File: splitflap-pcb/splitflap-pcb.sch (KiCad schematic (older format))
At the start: 21 parts, among them J1 INPUT CONN, J2 HALL 1, J3 HALL 2, J4 STEPPER 1, J5 STEPPER 2, J6 OUTPUT CONN, J7 AVR-ISP-6, U1 REGULATOR, U2 ATtiny88-AU, U3 TPIC6595

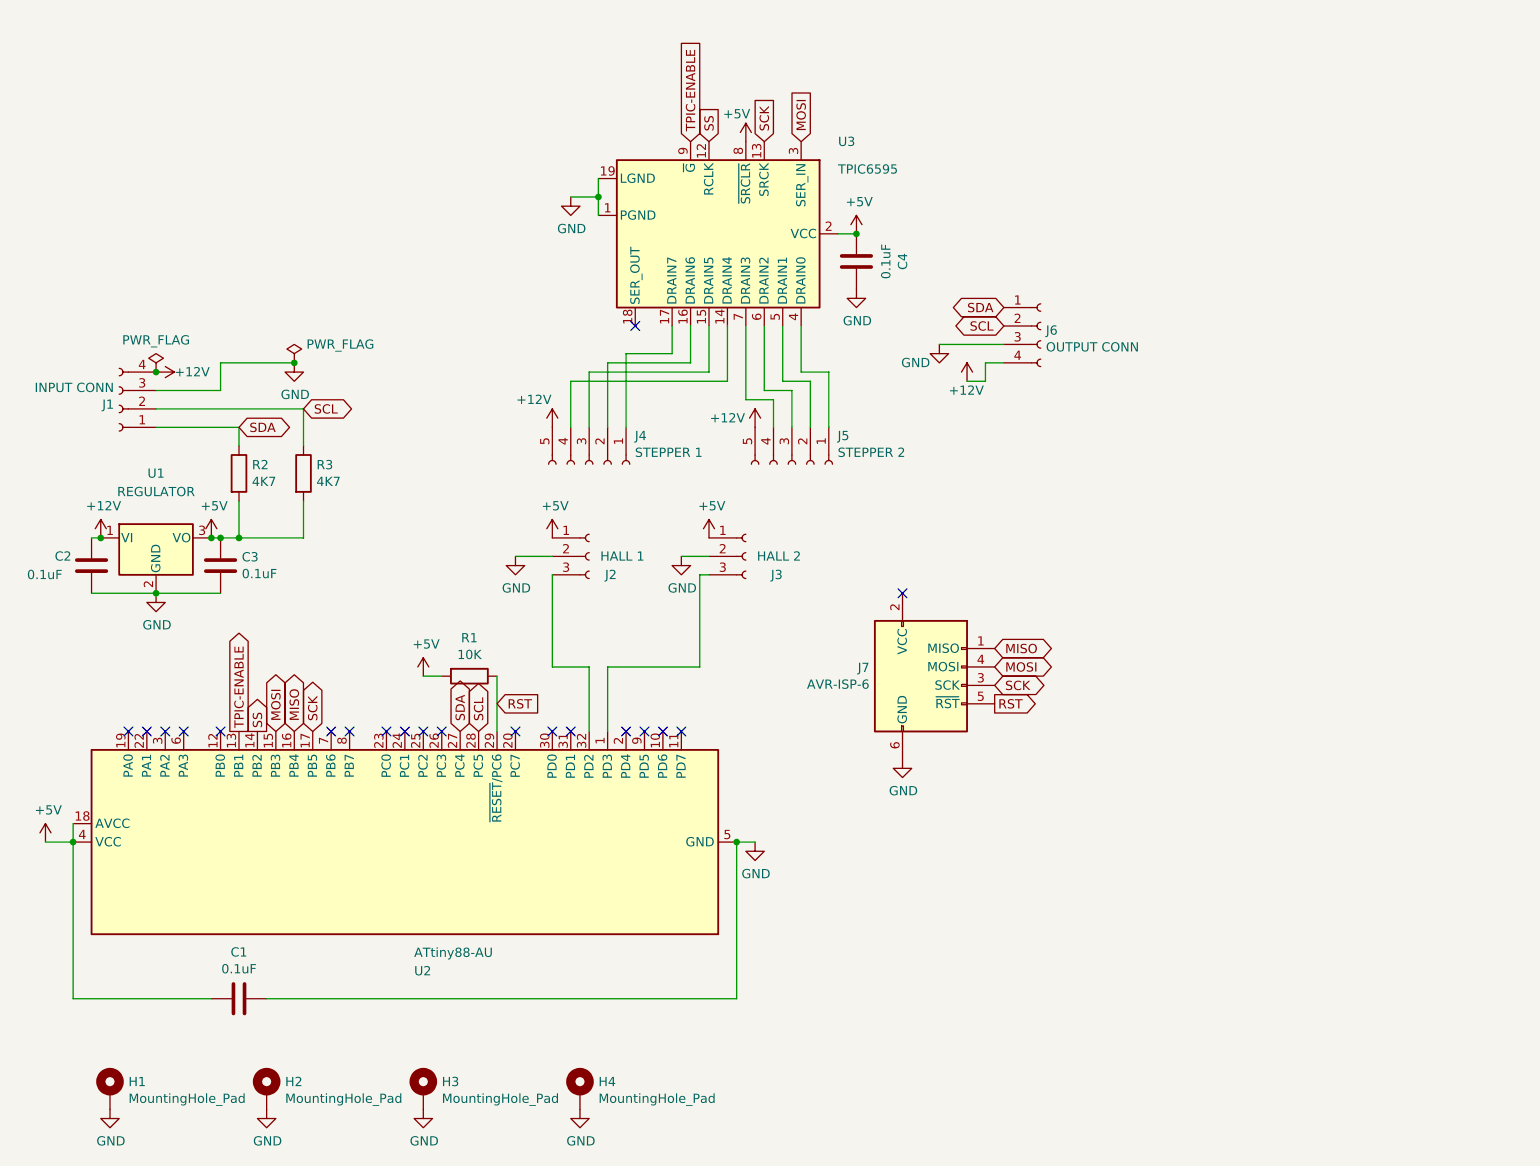
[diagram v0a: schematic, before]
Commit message: new netlist
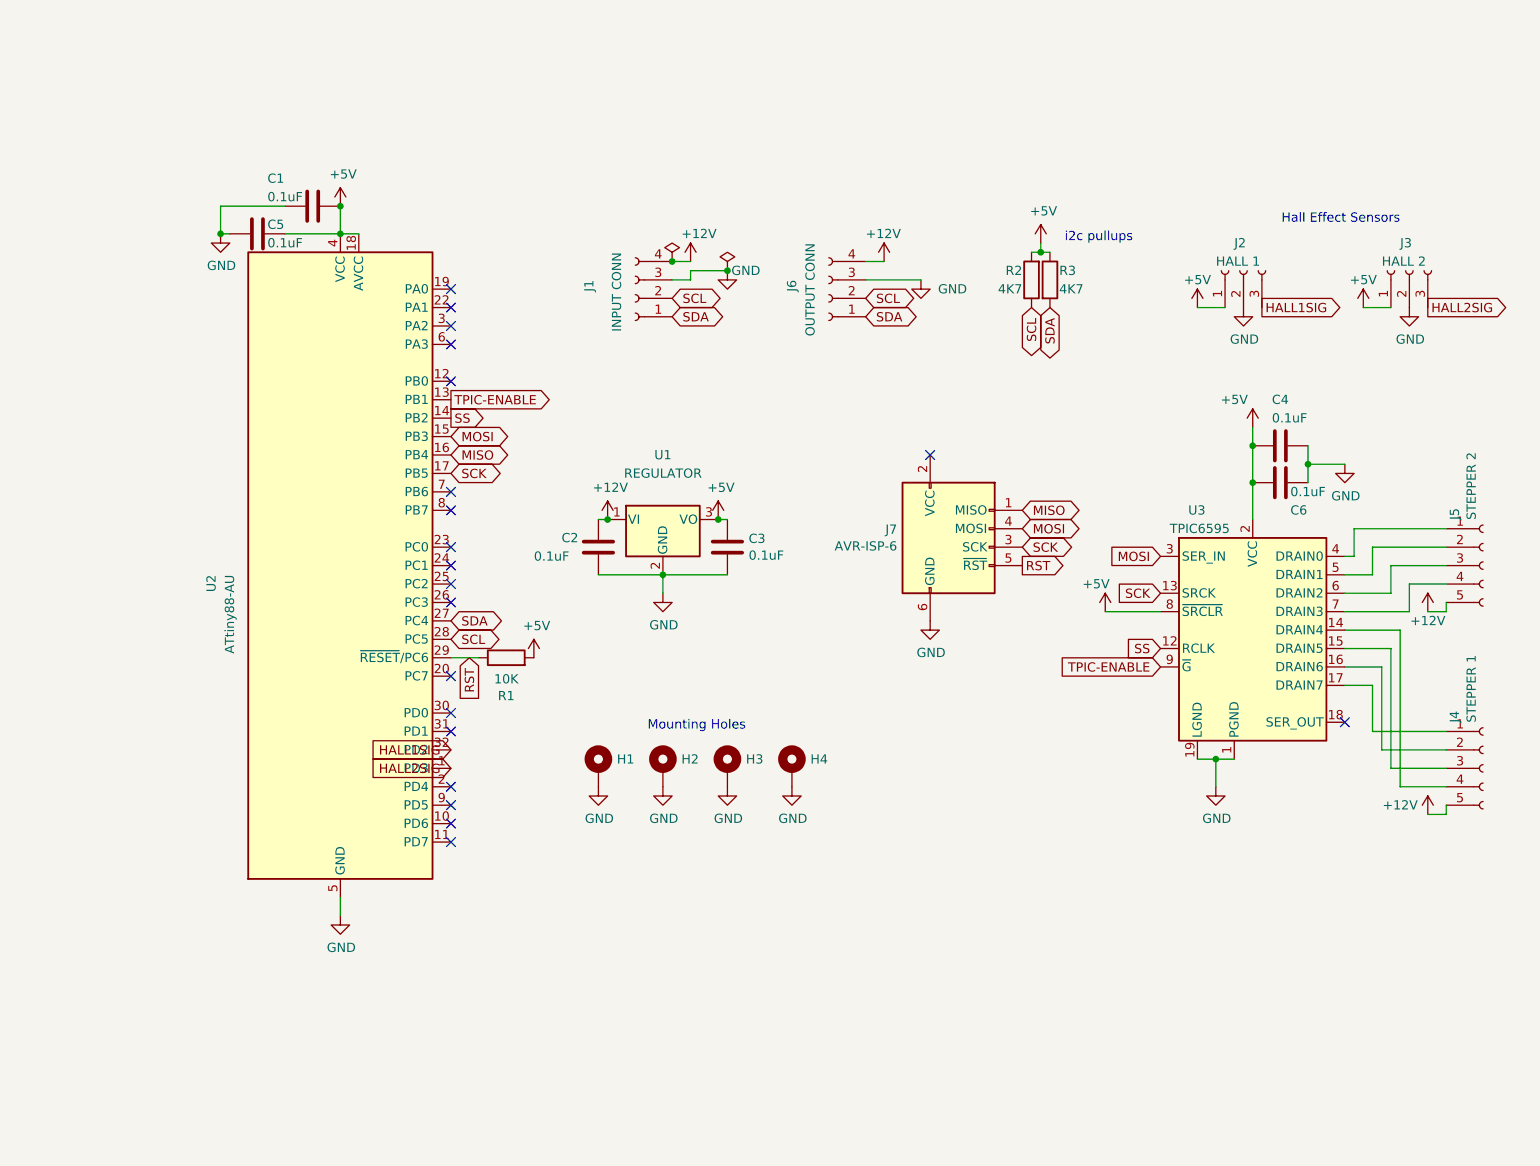
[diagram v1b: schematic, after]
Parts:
- added C5, C6: 0.1uF, Capacitor_SMD:C_0603_1608Metric, symbol Device:C
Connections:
- net +5V: now also C4.1, R3.1, C5.2, C6.1; no longer C4.2, R3.2
- net GND: now also C4.2, C5.1, C6.2; no longer C4.1
- net SCL: now also R2.1; no longer R3.1
- net SDA: now also R3.2; no longer R2.1
- net HALL2SIG: now reaches J3.3 (Pin_3), U2.1 (PD3)
- net HALL1SIG: now reaches J2.3 (Pin_3), U2.32 (PD2)
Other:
- note added: "Hall Effect Sensors"
- note added: "Mounting Holes"
- note added: "i2c pullups"
- moved on the sheet: C1, C2, C3, C4, H1, H2, H3, H4, J1, J2, J3, J4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

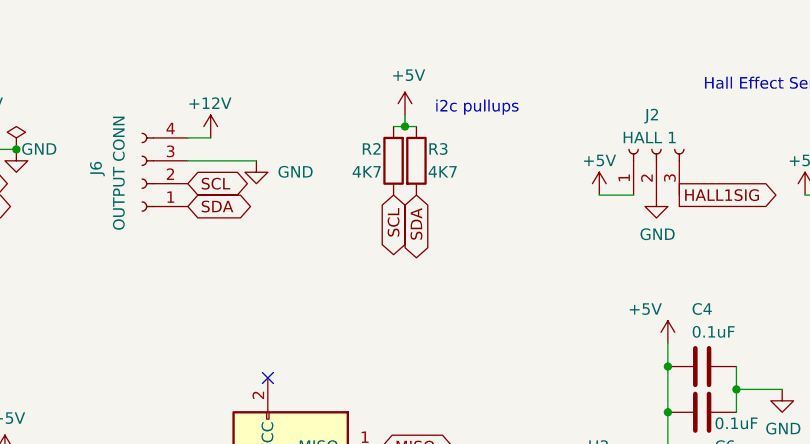
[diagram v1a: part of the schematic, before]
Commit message: More
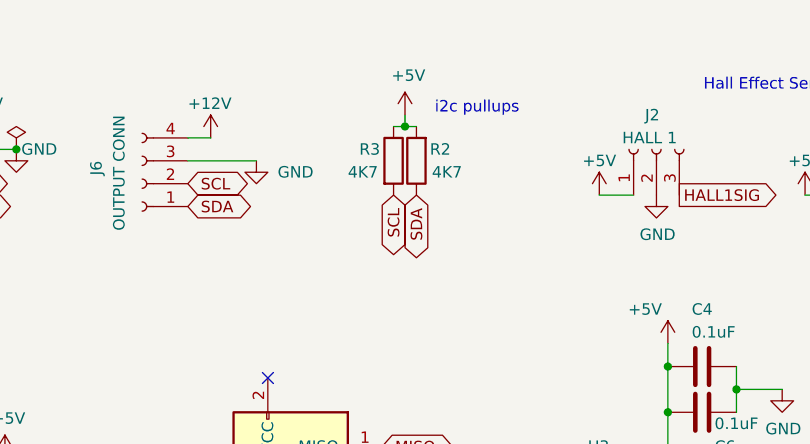
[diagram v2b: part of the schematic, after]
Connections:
- net SCL: now also R3.2; no longer R2.1
- net SDA: now also R2.1; no longer R3.2
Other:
- moved on the sheet: R2, R3
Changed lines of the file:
@@
 $EndComp
 $Comp
-L Device:R R2
-U 1 1 5CC6D9CB
+L Device:R R3
+U 1 1 5CC6DB71
 P 6050 1800
-F 0 "R2" H 6100 1750 50  0000 L CNN
-F 1 "4K7" H 6100 1850 50  0000 L CNN
+F 0 "R3" H 5900 1850 50  0000 L CNN
+F 1 "4K7" H 5850 1750 50  0000 L CNN
 F 2 "Resistor_SMD:R_0603_1608Metric" V 5980 1800 50  0001 C CNN
 F 3 "~" H 6050 1800 50  0001 C CNN
 	1    6050 1800
-	-1   0    0    1
-$EndComp
-$Comp
-L Device:R R3
-U 1 1 5CC6DB71
-P 6150 1800
-F 0 "R3" H 6200 1850 50  0000 L CNN
-F 1 "4K7" H 6200 1750 50  0000 L CNN
-F 2 "Resistor_SMD:R_0603_1608Metric" V 6080 1800 50  0001 C CNN
-F 3 "~" H 6150 1800 50  0001 C CNN
-	1    6150 1800
 	1    0    0    -1
 $EndComp
@@
 Wire Wire Line
 	7250 2900 7250 3100
+$Comp
+L Device:R R2
+U 1 1 5CC6D9CB
+P 6150 1800
+F 0 "R2" H 6000 1750 50  0000 L CNN
+F 1 "4K7" H 5950 1850 50  0000 L CNN
+F 2 "Resistor_SMD:R_0603_1608Metric" V 6080 1800 50  0001 C CNN
+F 3 "~" H 6150 1800 50  0001 C CNN
+	1    6150 1800
+	-1   0    0    1
+$EndComp
 $EndSCHEMATC
